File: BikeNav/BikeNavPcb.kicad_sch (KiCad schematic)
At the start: 3 parts, among them U1 TP4056, U2 ESP32-C3_SUPERMINI_TH

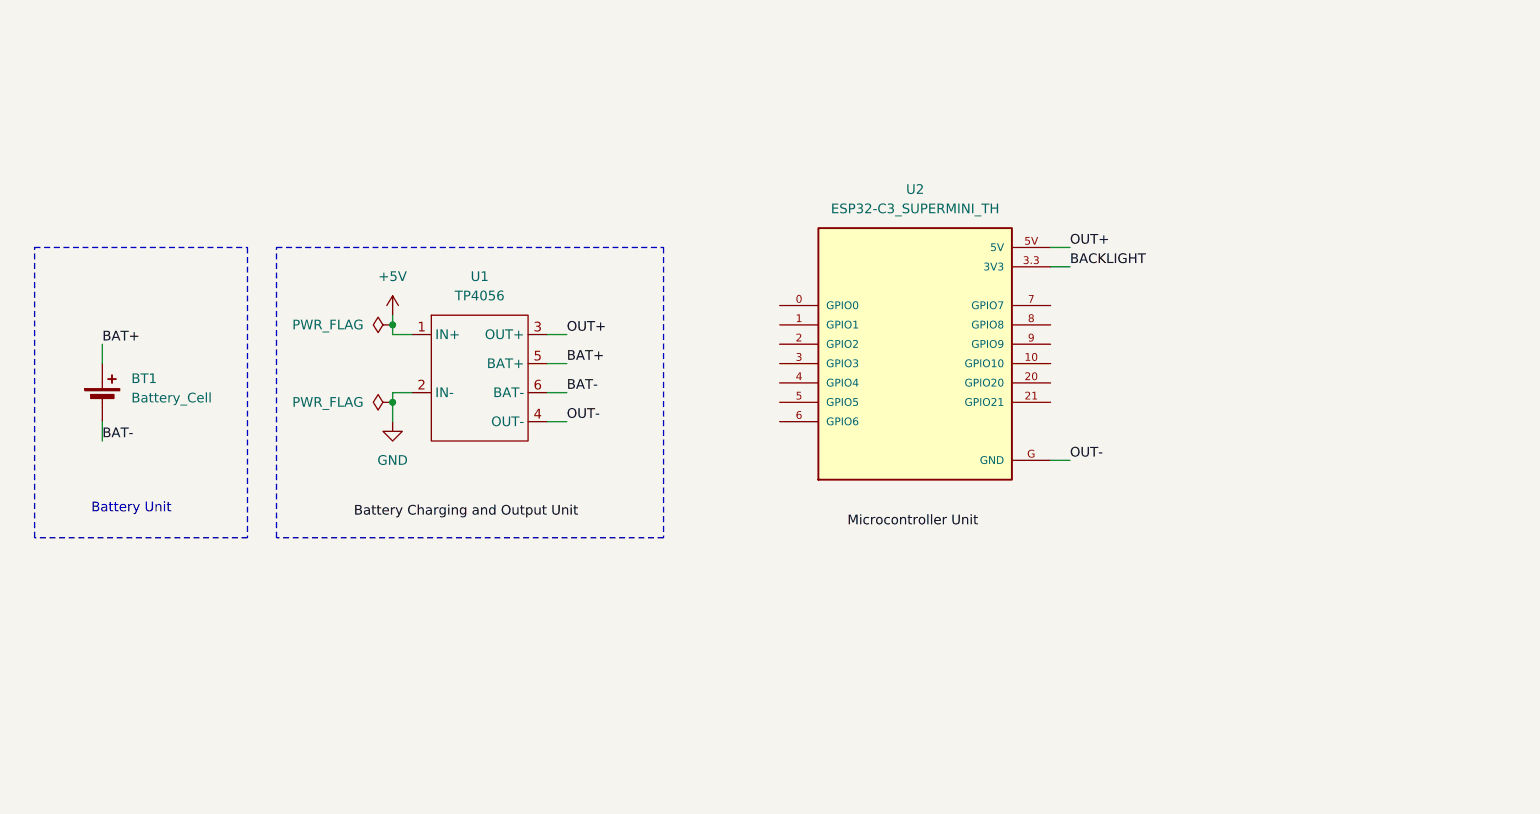
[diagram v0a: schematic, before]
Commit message: Update PCB Design
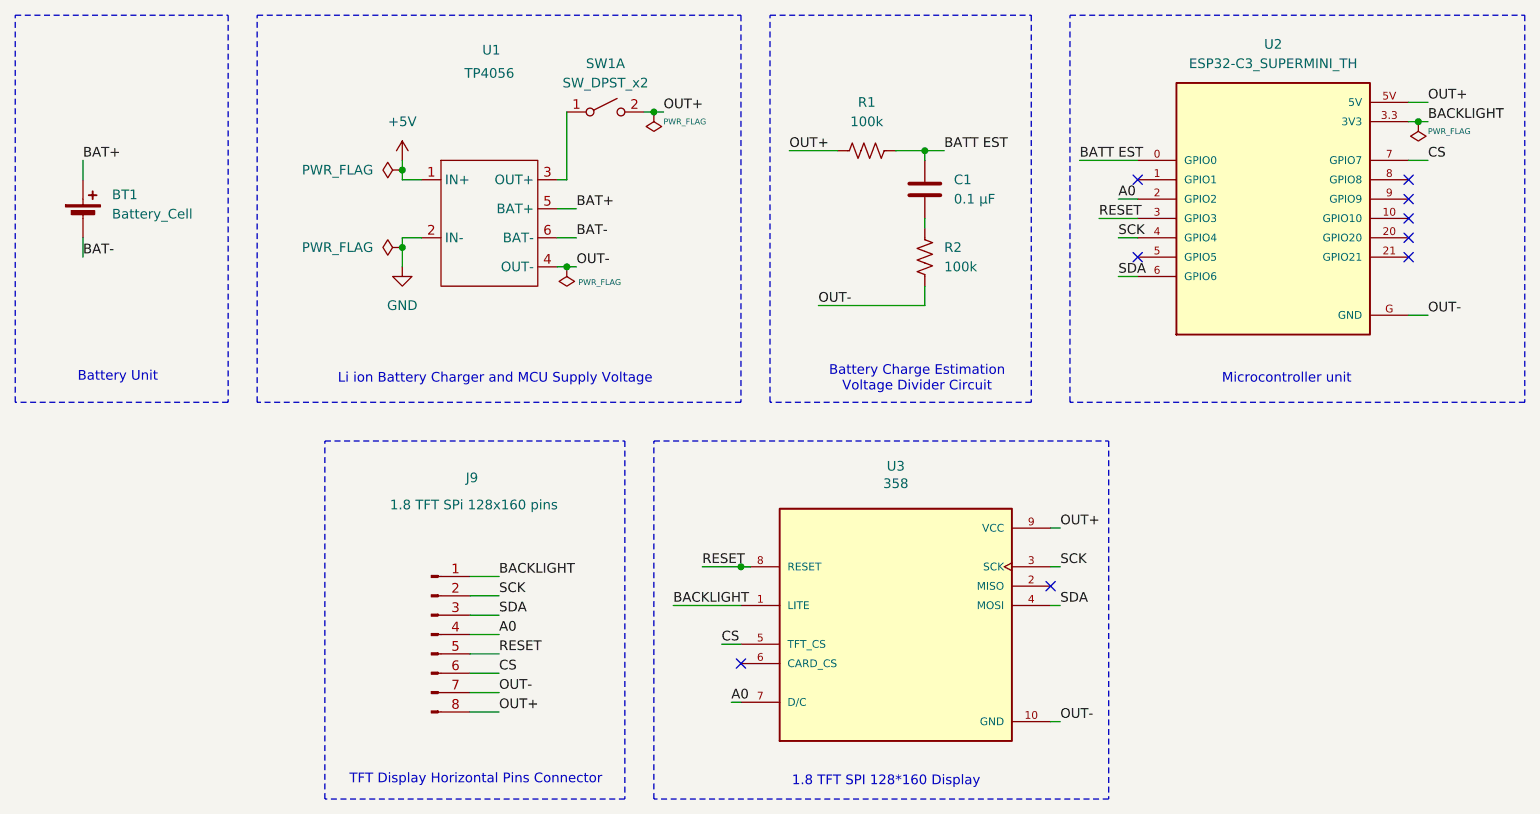
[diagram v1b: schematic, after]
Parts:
- added C1: 0.1 µF, Capacitor_THT:C_Disc_D10.0mm_W2.5mm_P5.00mm, symbol Device:C
- added J9: 1.8 TFT SPi 128x160 pins, Connector_PinSocket_2.54mm:PinSocket_1x08_P2.54mm_Vertical, symbol Connector:Conn_01x08_Pin
- added R1, R2: 100k, Resistor_THT:R_Axial_DIN0204_L3.6mm_D1.6mm_P5.08mm_Horizontal, symbol Device:R_US
- added SW1: SW_DPST_x2, Button_Switch_SMD:SW_DIP_SPSTx01_Slide_Copal_CHS-01A_W5.08mm_P1.27mm_JPin, symbol Switch:SW_DPST_x2
- added U3: 358, ST7735:ST7735, symbol ST7735:358
- U1: footprint Footprint:TP4056 -> TP4056:TP4056
- U2: footprint ESP32-C3_SUPERMINI_TH:MODULE_ESP32-C3_SUPERMINI_TH -> ESP32C3_Supermini_symbol_footprint:MODULE_ESP32-C3_SUPERMINI_TH
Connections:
- net BACKLIGHT: now also J9.1 (Pin_1), U3.1 (LITE)
- net OUT+: now also J9.8 (Pin_8), R1.2, SW1.2 (B), U3.9 (VCC); no longer U1.3 (OUT+)
- net OUT-: now also J9.7 (Pin_7), R2.2, U3.10 (GND)
- net BATT EST: now reaches U2.0 (GPIO0)
- net BATT EST: now also C1.1, R1.1
- net A0: now reaches U2.2 (GPIO2)
- net A0: now also J9.4 (Pin_4), U3.7 (D/C)
- net RESET: now reaches U2.3 (GPIO3)
- net RESET: now also J9.5 (Pin_5), U3.8 (RESET)
- net SCK: now reaches U2.4 (GPIO4)
- net SCK: now also J9.2 (Pin_2), U3.3 (SCK)
- net SDA: now reaches U2.6 (GPIO6)
- net SDA: now also J9.3 (Pin_3), U3.4 (MOSI)
- net CS: now reaches U2.7 (GPIO7)
- net CS: now also J9.6 (Pin_6), U3.5 (TFT_CS)
- new net: SW1.1 (A), U1.3 (OUT+)
- new net: C1.2, R2.1
- no-connect marks 0 -> 9
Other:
- note added: "1.8 TFT SPI 128*160 Display"
- note added: "Battery Charge Estimation Voltage Divider Circuit"
- note added: "Li ion Battery Charger and MCU Supply Voltage"
- note added: "Microcontroller unit"
- note added: "TFT Display Horizontal Pins Connector"
- moved on the sheet: BT1, U1, U2
